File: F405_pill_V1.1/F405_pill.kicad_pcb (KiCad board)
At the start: 4 copper layers, 54.1 x 26.6 mm, 77 parts, among them J1 Conn_01x04_Male, J2 Conn_01x04_Male, J4 TYPE-C-31-M-12, J5 Conn_01x02, U1 STM32F405RGTx, U2 TJA1050T/CM,118, U3 LM1117-3.3, U4 STM32F405_pill, U5 HT7550, U6 BMI160, U7 MPU-9250, U8 LSM6DS3, U9 BMI270, Y1 8MHz

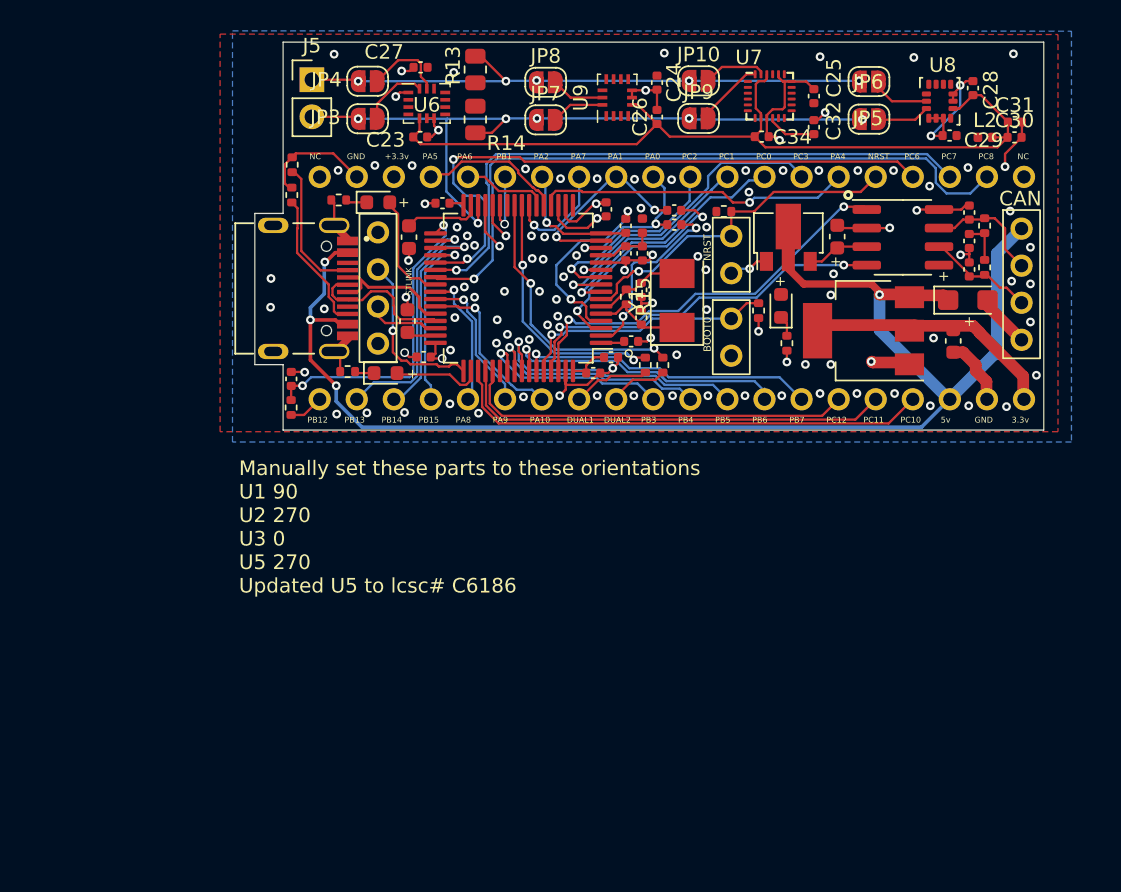
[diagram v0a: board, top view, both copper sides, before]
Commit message: add MCU
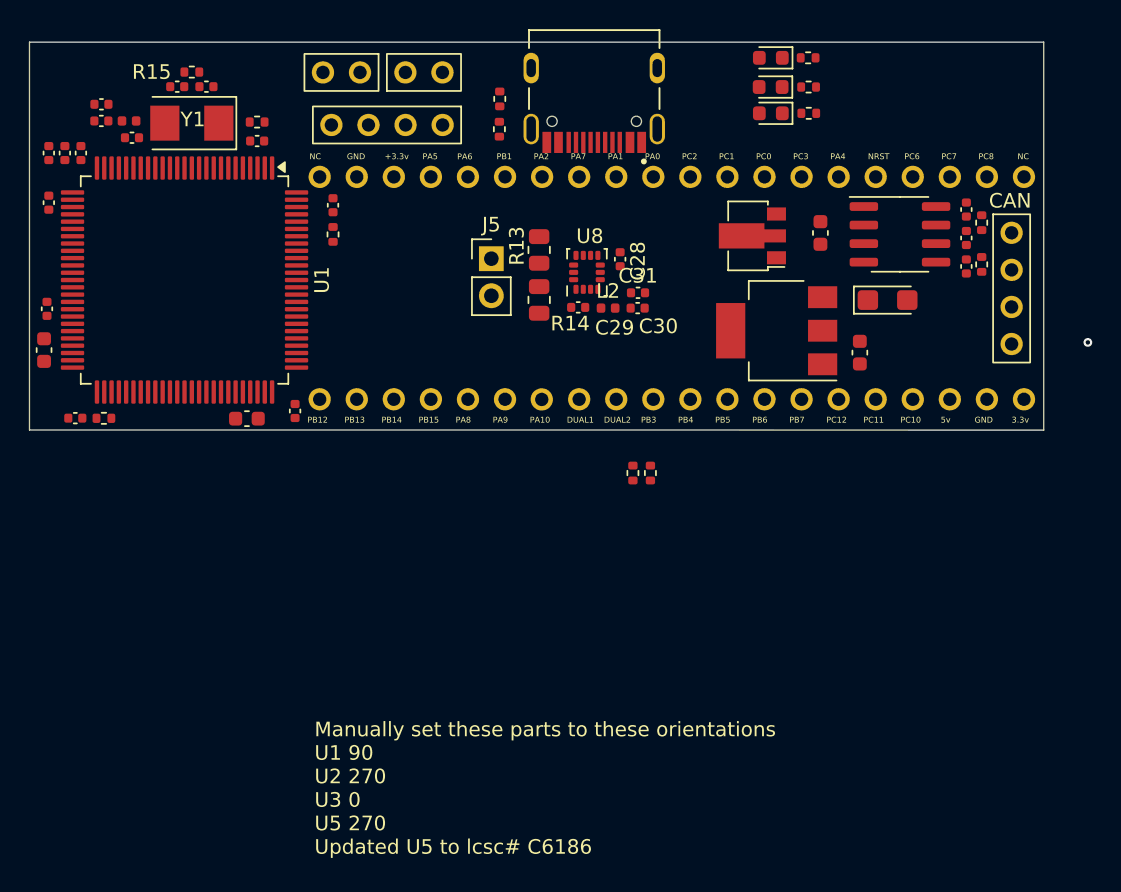
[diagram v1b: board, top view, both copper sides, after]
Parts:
- removed C23, C24, C25, C26, C27, C32, C34: 100n, Capacitor_SMD:C_0402_1005Metric
- removed JP10, JP4, JP6, JP8: SCL, Jumper:SolderJumper-2_P1.3mm_Open_RoundedPad1.0x1.5mm
- removed JP3, JP5, JP7, JP9: SDA, Jumper:SolderJumper-2_P1.3mm_Open_RoundedPad1.0x1.5mm
- removed U6: BMI160, Package_LGA:Bosch_LGA-14_3x2.5mm_P0.5mm
- removed U7: MPU-9250, Sensor_Motion:InvenSense_QFN-24_3x3mm_P0.4mm
- removed U9: BMI270, Package_LGA:Bosch_LGA-14_3x2.5mm_P0.5mm
- U1: value STM32F405RGTx -> STM32F405VGTx; footprint Package_QFP:LQFP-64_10x10mm_P0.5mm -> Package_QFP:LQFP-100_14x14mm_P0.5mm
- U2: value TJA1050T/CM,118 -> TJA1050T/CM,118
- moved C18 41.9 mm to (81.4, 75.4), turned to -90 degrees
- moved C17 41.0 mm to (82.5, 75.4), turned to -90 degrees
- moved C19 39.8 mm to (80.3, 75.4)
- moved C5 38.2 mm to (83.9, 73.2), turned to 180 degrees
- moved C12 37.7 mm to (80.2, 86.1), turned to 90 degrees
- moved C8 37.3 mm to (83.9, 72.1), turned to 180 degrees
- moved R5 37.1 mm to (132.4, 70.9), turned to 180 degrees
- moved L1 35.9 mm to (85.8, 73.2), turned to 180 degrees
- moved Y1 35.4 mm to (90.1, 73.4), turned to 180 degrees
- moved C6 34.7 mm to (89.1, 70.9), turned to 180 degrees
- moved C3 33.7 mm to (91.1, 70.9), turned to 0 degrees
- moved R15 33.5 mm to (90.1, 69.9), turned to 0 degrees
- moved D2 32.9 mm to (129.8, 70.9), turned to 180 degrees
- moved C4 32.9 mm to (86.0, 74.4), turned to 180 degrees
- moved R7 32.8 mm to (132.4, 72.7), turned to 180 degrees
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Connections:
- U1 pad 1: +3V3 -> unconnected-(U1-PE2-Pad1)
- U1 pad 10: PC2 -> GND
- U1 pad 11: PC3 -> +3V3
- U1 pad 12: GND -> Net-(U1-PH0)
- U1 pad 13: +3.3VA -> Net-(U1-PH1)
- U1 pad 14: PA0 -> NRST
- U1 pad 15: PA1 -> PC0
- U1 pad 16: PA2 -> PC1
- U1 pad 17: PA3 -> PC2
- U1 pad 18: GND -> PC3
- U1 pad 2: PC13 -> unconnected-(U1-PE3-Pad2)
- U1 pad 20: PA4 -> GND
- U1 pad 21: PA5 -> +3.3VA
- U1 pad 22: PA6 -> +3.3VA
- U1 pad 23: PA7 -> PA0
- U1 pad 24: PC4 -> PA1
- U1 pad 25: PC5 -> PA2
- U1 pad 26: PB0 -> PA3
- U1 pad 27: PB1 -> GND
- U1 pad 28: GND -> +3V3
- U1 pad 29: PB10 -> PA4
- U1 pad 3: PC14 -> unconnected-(U1-PE4-Pad3)
- U1 pad 30: PB11 -> PA5
- U1 pad 31: Net-(U1-VCAP_1) -> PA6
- U1 pad 32: +3V3 -> PA7
- U1 pad 33: PB12 -> PC4
- U1 pad 34: PB13 -> PC5
- U1 pad 35: PB14 -> PB0
- U1 pad 36: PB15 -> PB1
- U1 pad 37: PC6 -> GND
- U1 pad 38: PC7 -> unconnected-(U1-PE7-Pad38)
- U1 pad 39: PC8 -> unconnected-(U1-PE8-Pad39)
- U1 pad 4: PC15 -> unconnected-(U1-PE5-Pad4)
- U1 pad 40: PC9 -> unconnected-(U1-PE9-Pad40)
- U1 pad 41: PA8 -> unconnected-(U1-PE10-Pad41)
- U1 pad 42: PA9 -> unconnected-(U1-PE11-Pad42)
- U1 pad 43: PA10 -> unconnected-(U1-PE12-Pad43)
- U1 pad 44: USB_D- -> unconnected-(U1-PE13-Pad44)
- U1 pad 45: USB_D+ -> unconnected-(U1-PE14-Pad45)
- U1 pad 46: SWDIO -> unconnected-(U1-PE15-Pad46)
- U1 pad 47: Net-(U1-VCAP_2) -> PB10
- U1 pad 48: +3V3 -> PB11
- U1 pad 49: SWCLK -> Net-(U1-VCAP_1)
- U1 pad 5: Net-(U1-PH0) -> unconnected-(U1-PE6-Pad5)
- U1 pad 50: PA15 -> +3V3
- U1 pad 51: PC10 -> PB12
- U1 pad 52: PC11 -> PB13
- U1 pad 53: PC12 -> PB14
- U1 pad 54: PD2 -> PB15
- U1 pad 55: PB3 -> unconnected-(U1-PD8-Pad55)
- U1 pad 56: PB4 -> unconnected-(U1-PD9-Pad56)
- U1 pad 57: PB5 -> unconnected-(U1-PD10-Pad57)
- U1 pad 58: PB6 -> unconnected-(U1-PD11-Pad58)
- U1 pad 59: PB7 -> unconnected-(U1-PD12-Pad59)
- U1 pad 6: Net-(U1-PH1) -> +3V3
- U1 pad 60: Net-(JP1-B) -> unconnected-(U1-PD13-Pad60)
- U1 pad 61: PB8 -> unconnected-(U1-PD14-Pad61)
- U1 pad 62: PB9 -> unconnected-(U1-PD15-Pad62)
- U1 pad 63: GND -> PC6
- U1 pad 64: +3V3 -> PC7
- U1 pad 7: NRST -> PC13
- U1 pad 8: PC0 -> PC14
- U1 pad 9: PC1 -> PC15
- U8 pad 13: Net-(JP6-B) -> PB10
- U8 pad 14: Net-(JP5-B) -> PB11
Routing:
- net GND: track 95.0 -> 0.00 mm, vias 100 -> 0
- net +5V: track 94.2 -> 0.00 mm, vias 4 -> 0
- net 3.3F: track 58.3 -> 0.00 mm
- net PB10: track 56.1 -> 0.00 mm, vias 6 -> 0
- net PB11: track 49.8 -> 0.00 mm, vias 6 -> 0
- net PC8: track 47.6 -> 0.00 mm, vias 1 -> 0
- net PC6: track 43.3 -> 0.00 mm, vias 2 -> 0
- net PC7: track 42.8 -> 0.00 mm, vias 1 -> 0
- net PC10: track 33.2 -> 0.00 mm
- net PC11: track 30.1 -> 0.00 mm
- net +3V3: track 29.9 -> 0.00 mm, vias 12 -> 1
- net PB9: track 27.8 -> 0.00 mm, vias 2 -> 0
- net PC12: track 27.0 -> 0.00 mm
- net PB8: track 26.2 -> 0.00 mm, vias 2 -> 0
- net NRST: track 23.6 -> 0.00 mm, vias 1 -> 0
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- removed copper zone on B.Cu, net +3V3
- removed copper zone on F.Cu, net +3V3
- removed copper zone on In1.Cu, net GND
- removed copper zone on In2.Cu, net GND
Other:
- board size 54.1 x 26.6 mm -> 69.5 x 26.6 mm
- board text added: "STM32F405VG PILL V1.2"
- board text removed: "+"
- board text removed: "+5v"
- board text removed: "3V3"
- board text removed: "BOOT0"
- board text removed: "CAN_H"
- board text removed: "CAN_L"
- board text removed: "LICENSE: BSD"
- board text removed: "STLINK"
- board text removed: "STM32F405RG PILL V1.1"
- board text removed: "SWCLK"
- board text removed: "SWDIO"
